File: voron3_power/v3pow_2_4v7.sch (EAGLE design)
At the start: 54 parts, among them Q1 IRF3205, Q2 IRF3205, Q3 IRF3205, Q4 IRF3205

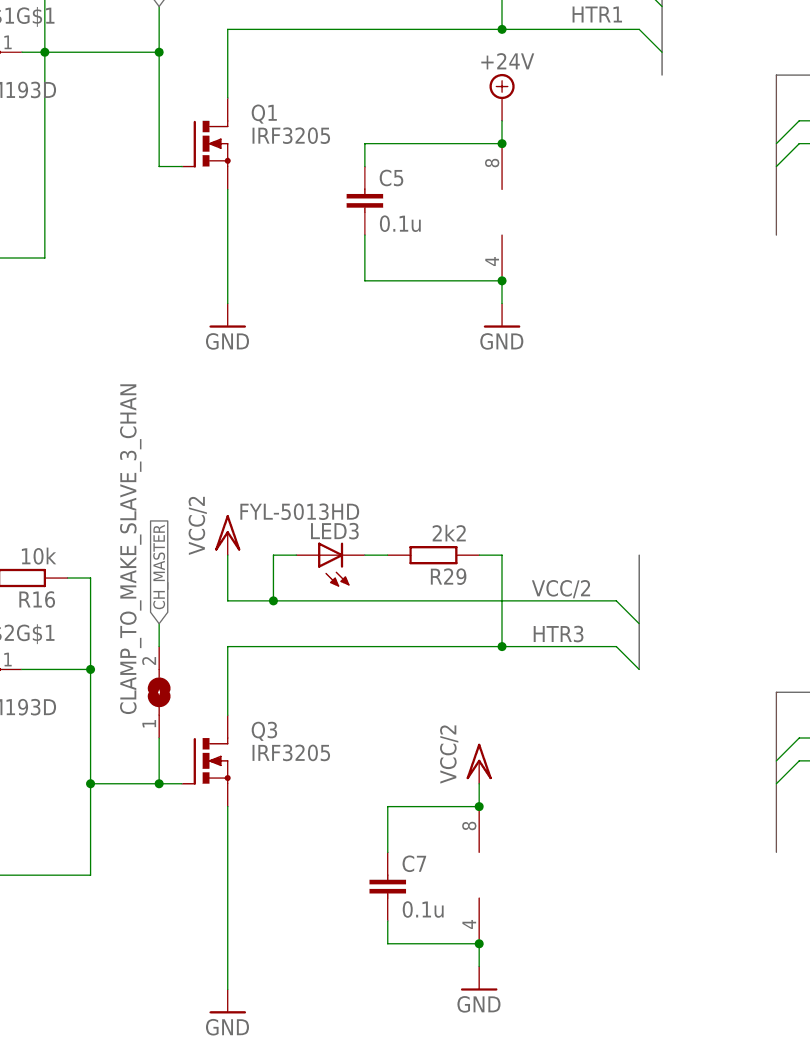
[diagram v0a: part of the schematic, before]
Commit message: capacitor chan, and all done
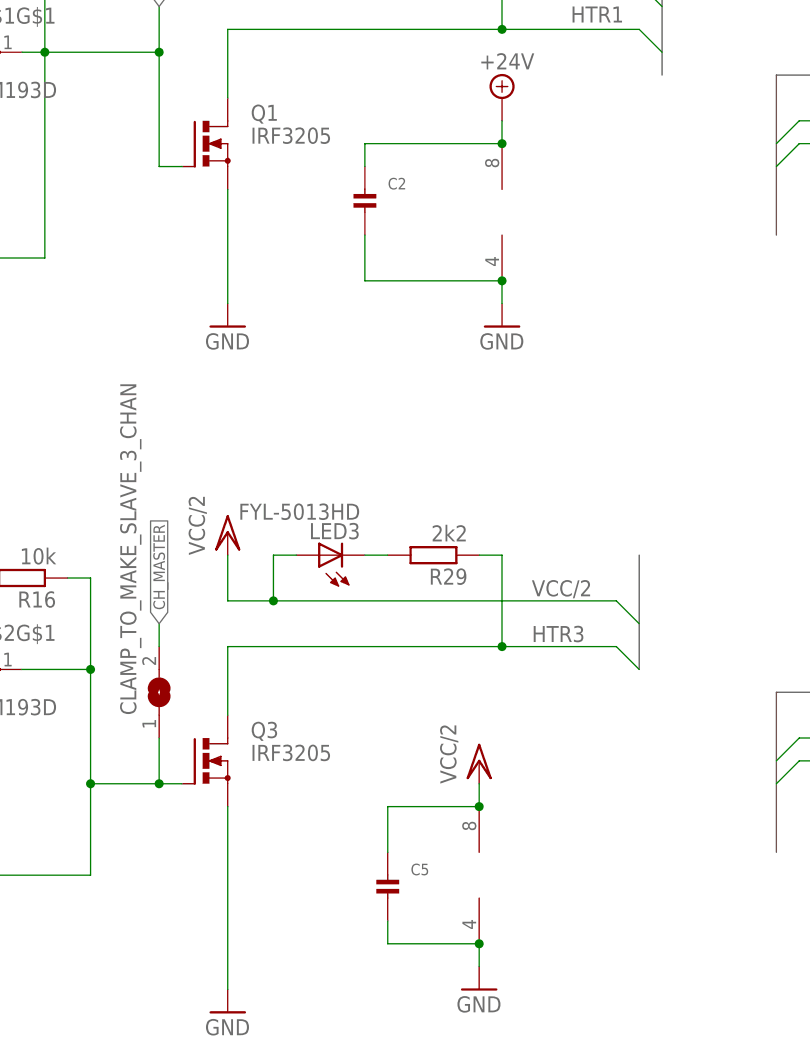
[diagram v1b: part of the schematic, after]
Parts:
- removed C7: 0.1u, rcl:C-EUC0805
- added C2: (no value), microbuilder:CAP_CERAMIC1206
- C5: value 0.1u -> (none); device rcl:C-EUC0805 -> microbuilder:CAP_CERAMIC1206
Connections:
- net +24V: now also C2.P$1; no longer C5.1
- net GND: now also C2.P$2, C5.P$2; no longer C5.2, C7.2
- net VCC/2: now also C5.P$1; no longer C7.1
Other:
- moved on the sheet: C5
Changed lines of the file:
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@@
 <part name="GND14" library="supply1" deviceset="GND" device=""/>
 <part name="P+9" library="supply1" deviceset="VCC/2" device=""/>
-<part name="C7" library="rcl" deviceset="C-EU" device="C0805" value="0.1u"/>
 <part name="SUPPLY9" library="supply2" deviceset="+24V" device=""/>
-<part name="C5" library="rcl" deviceset="C-EU" device="C0805" value="0.1u"/>
 <part name="X_220IN" library="con-wago_2706" deviceset="2706-102" device=""/>
 <part name="CLAMP_TO_MAKE_SLAVE_2_CHAN" library="jumper" deviceset="SJ" device=""/>
@@
 <part name="SUPPLY7" library="supply2" deviceset="+24V" device=""/>
 <part name="P+7" library="supply1" deviceset="VCC/2" device=""/>
+<part name="C2" library="microbuilder" deviceset="CAP_CERAMIC" device="1206"/>
+<part name="C5" library="microbuilder" deviceset="CAP_CERAMIC" device="1206"/>
 </parts>
 <sheets>
@@
 <instance part="GND14" gate="1" x="203.2" y="144.78" rot="R270"/>
 <instance part="P+9" gate="G$1" x="226.06" y="15.24"/>
-<instance part="C7" gate="G$1" x="215.9" y="2.54"/>
 <instance part="SUPPLY9" gate="+24V" x="228.6" y="88.9"/>
-<instance part="C5" gate="G$1" x="213.36" y="78.74"/>
 <instance part="X_220IN" gate="G$1" x="137.16" y="167.64" rot="R180"/>
 <instance part="CLAMP_TO_MAKE_SLAVE_2_CHAN" gate="1" x="345.44" y="93.98" rot="R90"/>
@@
 <instance part="SUPPLY7" gate="+24V" x="190.5" y="149.86" rot="R90"/>
 <instance part="P+7" gate="G$1" x="190.5" y="160.02" rot="R90"/>
+<instance part="C2" gate="G$1" x="213.36" y="76.2"/>
+<instance part="C5" gate="G$1" x="215.9" y="0"/>
 </instances>
 <busses>
@@
 <pinref part="U$1" gate="G$3" pin="V+"/>
 <wire x1="228.6" y1="86.36" x2="228.6" y2="83.82" width="0.1524" layer="91"/>
-<pinref part="C5" gate="G$1" pin="1"/>
 <wire x1="213.36" y1="81.28" x2="213.36" y2="83.82" width="0.1524" layer="91"/>
 <wire x1="213.36" y1="83.82" x2="228.6" y2="83.82" width="0.1524" layer="91"/>
 <junction x="228.6" y="83.82"/>
+<pinref part="C2" gate="G$1" pin="P$1"/>
 </segment>
 <segment>
@@
 <pinref part="U$1" gate="G$3" pin="V-"/>
 <wire x1="228.6" y1="68.58" x2="228.6" y2="66.04" width="0.1524" layer="91"/>
-<pinref part="C5" gate="G$1" pin="2"/>
 <wire x1="228.6" y1="68.58" x2="213.36" y2="68.58" width="0.1524" layer="91"/>
 <wire x1="213.36" y1="68.58" x2="213.36" y2="73.66" width="0.1524" layer="91"/>
 <junction x="228.6" y="68.58"/>
+<pinref part="C2" gate="G$1" pin="P$2"/>
 </segment>
 <segment>
@@
 <pinref part="U$2" gate="G$3" pin="V-"/>
 <wire x1="226.06" y1="-7.62" x2="226.06" y2="-5.08" width="0.1524" layer="91"/>
-<pinref part="C7" gate="G$1" pin="2"/>
 <wire x1="226.06" y1="-5.08" x2="215.9" y2="-5.08" width="0.1524" layer="91"/>
 <wire x1="215.9" y1="-5.08" x2="215.9" y2="-2.54" width="0.1524" layer="91"/>
 <junction x="226.06" y="-5.08"/>
+<pinref part="C5" gate="G$1" pin="P$2"/>
 </segment>
 <segment>
@@
 <pinref part="U$2" gate="G$3" pin="V+"/>
 <wire x1="226.06" y1="12.7" x2="226.06" y2="10.16" width="0.1524" layer="91"/>
-<pinref part="C7" gate="G$1" pin="1"/>
 <wire x1="226.06" y1="10.16" x2="215.9" y2="10.16" width="0.1524" layer="91"/>
 <wire x1="215.9" y1="10.16" x2="215.9" y2="5.08" width="0.1524" layer="91"/>
 <junction x="226.06" y="10.16"/>
-</segment>
-<segment>
+<pinref part="C5" gate="G$1" pin="P$1"/>
+</segment>
+<segment>
